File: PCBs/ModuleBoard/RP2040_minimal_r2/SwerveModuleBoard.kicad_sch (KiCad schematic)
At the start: 57 parts, among them IC1 AS5600-ASOT, J1 USB_B_Micro, J3 Conn_02x08_Odd_Even_MountingP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, J4 Conn_01x07, J5 Conn_01x06_Pin, J6 Conn_01x02, J7 Conn_01x06_Pin, J8 Conn_01x06, U2 W25Q128JVS, U3 RP2040, U4 DRV8245HQRXZRQ1, U5 DRV8245HQRXZRQ1, U6 MIC5219-3.3YM5, Y1 ABM8-272-T3

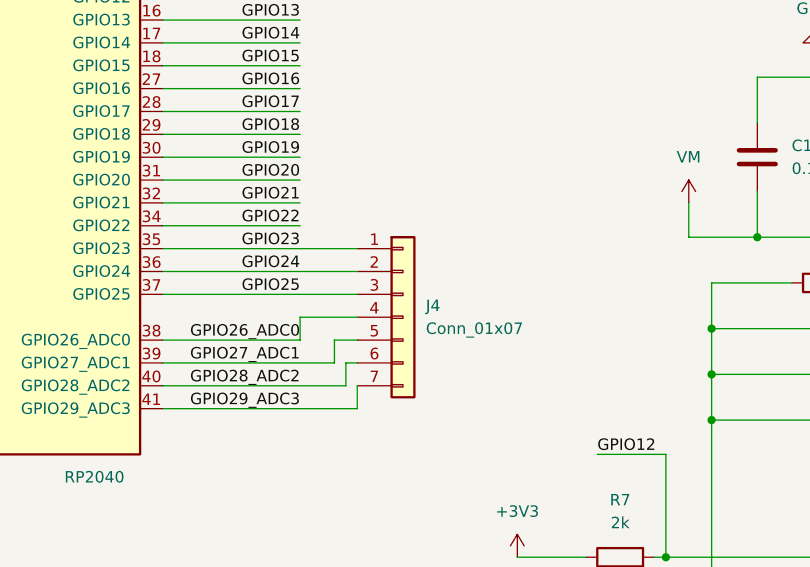
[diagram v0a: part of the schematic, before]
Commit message: vault backup: 2025-04-25 03:17:35
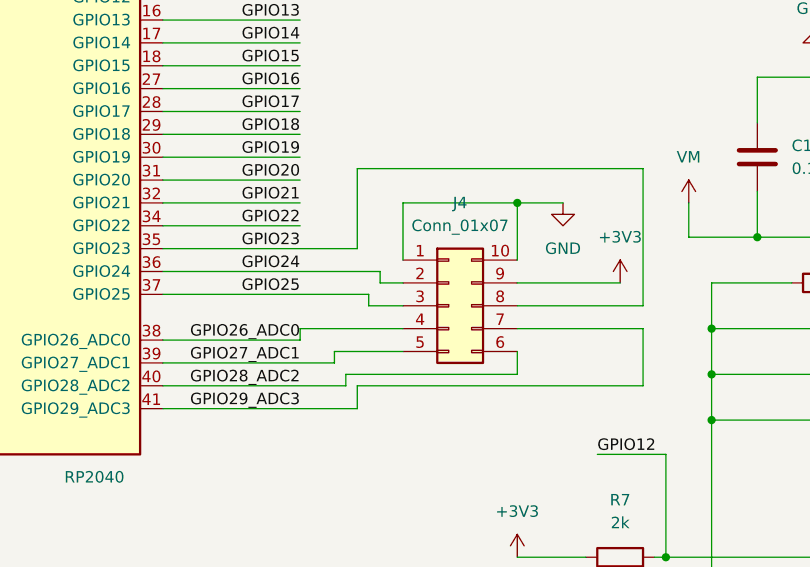
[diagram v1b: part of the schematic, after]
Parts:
- J4: footprint Connector_PinSocket_2.54mm:PinSocket_1x07_P2.54mm_Vertical -> Connector_PinHeader_2.54mm:PinHeader_2x05_P2.54mm_Vertical; symbol Connector_Generic:Conn_01x07 -> Connector_Generic:Conn_02x05_Counter_Clockwise
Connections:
- net +3V3: now also J4.9 (Pin_9)
- net GND: now also J4.1 (Pin_1), J4.10 (Pin_10)
- net GPIO23: now also J4.8 (Pin_8); no longer J4.1 (Pin_1)
